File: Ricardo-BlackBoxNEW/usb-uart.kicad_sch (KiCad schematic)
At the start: 12 parts, among them IC2 CP2102N-A02-GQFN24, J2 USB_C_Receptacle_USB2.0

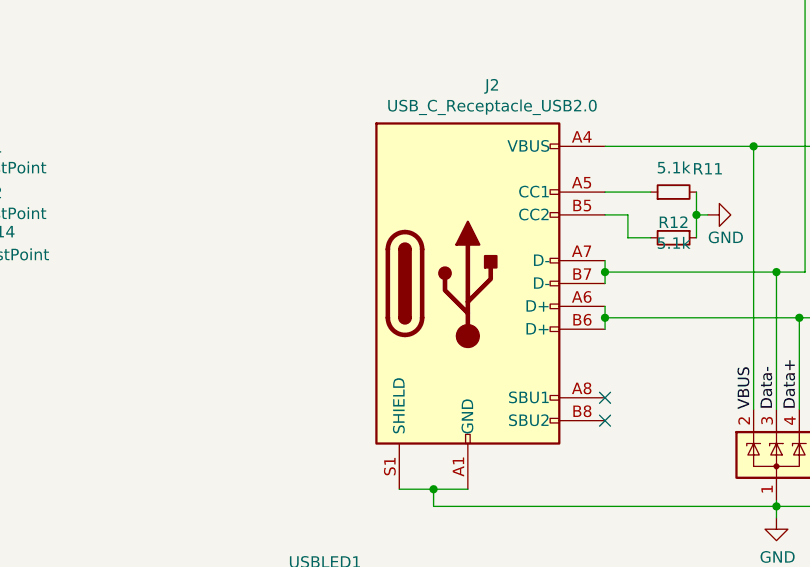
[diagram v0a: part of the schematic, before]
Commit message: RicardoBlackBox03_06_2023
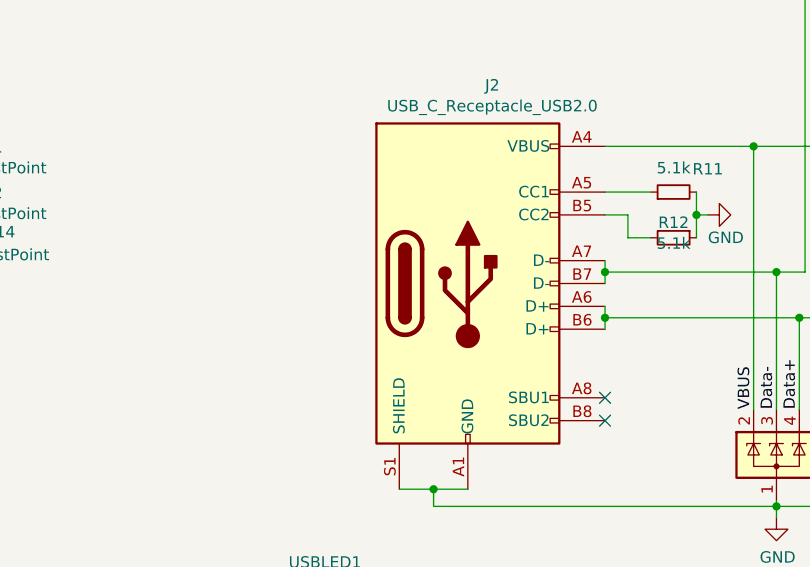
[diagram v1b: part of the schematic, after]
